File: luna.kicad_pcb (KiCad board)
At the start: 2 copper layers, 85 x 83.8 mm, 31 parts, among them J1 Conn_01x06_Male, J2 Conn_02x12_Top_Bottom, J3 Conn_01x02_Male, J4 Conn_01x02_Male, J5 Screw_Terminal_01x06, Q1 2N7002, Q2 2N7002, Q3 2N7002, Q4 DMN3404L, Q5 DMN3404L, Q6 DMN3404L, U1 LD1117S33TR_SOT223, U2 ESP32-WROOM-32

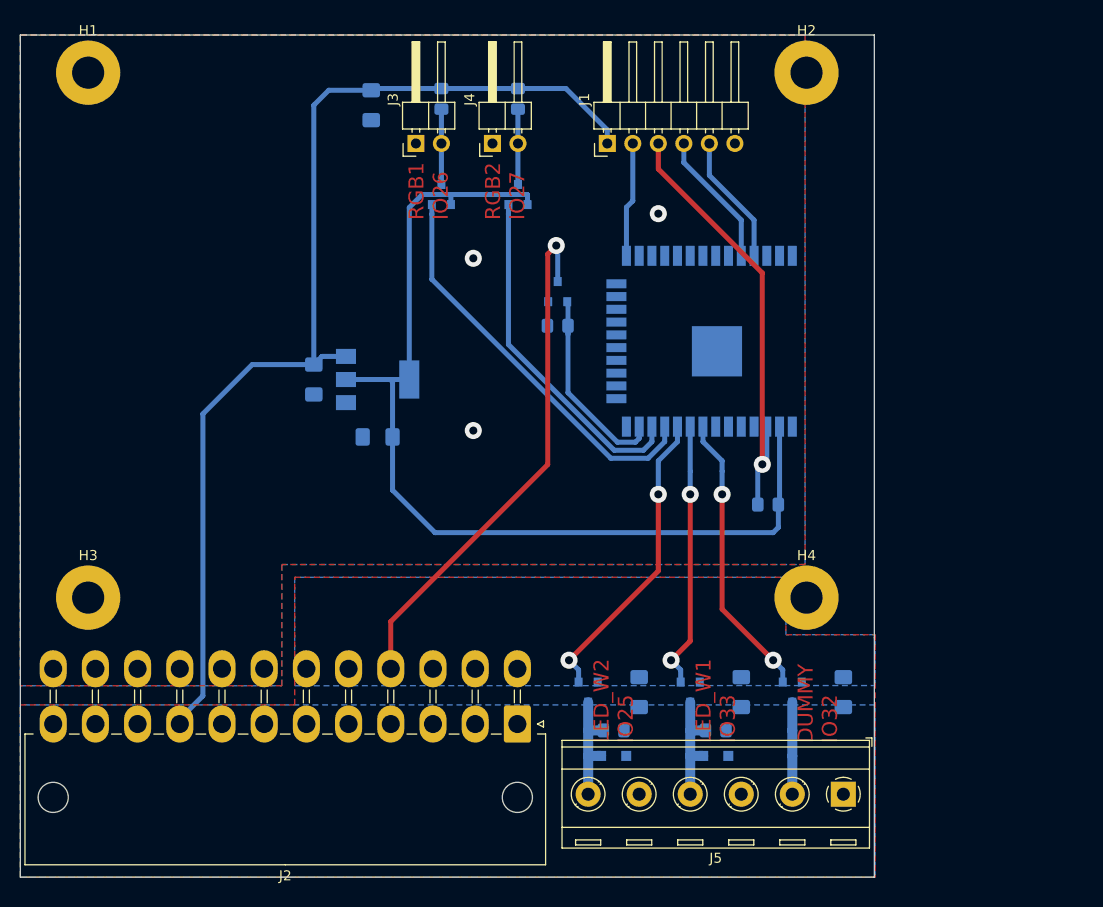
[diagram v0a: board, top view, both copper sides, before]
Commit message: Design in progress.
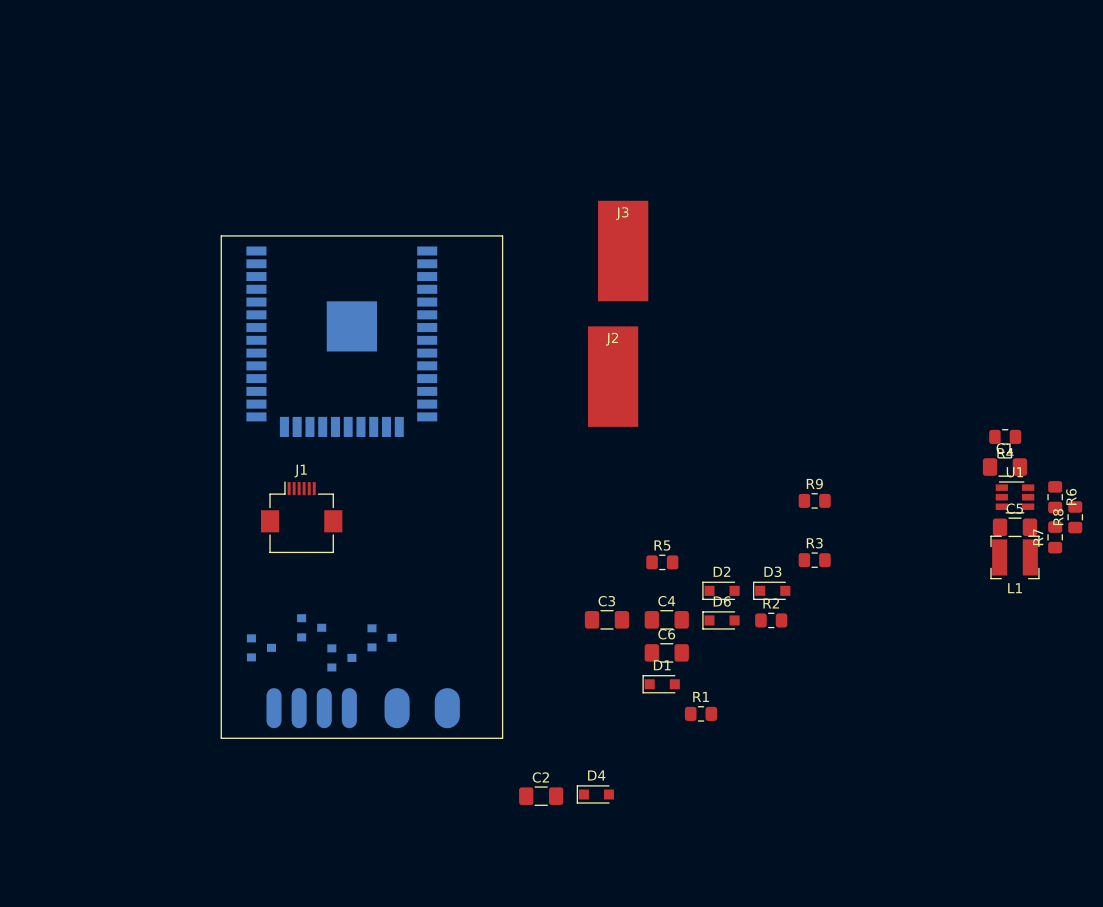
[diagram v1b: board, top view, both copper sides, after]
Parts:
- removed H1, H2, H3, H4: MountingHole_Pad, MountingHole:MountingHole_3.2mm_M3_Pad
- removed J4: Conn_01x02_Male, Connector_PinHeader_2.54mm:PinHeader_1x02_P2.54mm_Horizontal
- removed J5: Screw_Terminal_01x06, TerminalBlock_RND:TerminalBlock_RND_205-00291_1x06_P5.08mm_Horizontal
- removed Q5, Q6: DMN3404L, Package_TO_SOT_SMD:SOT-23
- added D3: D_Schottky, Diode_SMD:D_SOD-323_HandSoldering, F.Cu at (74.9, 55.3)
- added D4: D_Schottky, Diode_SMD:D_SOD-323_HandSoldering, F.Cu at (57.3, 75.6)
- added D5: LED_AGRB, custom:LED_STRIP_RGB, B.Cu at (29.0, 67.0)
- added D6: D_Schottky, Diode_SMD:D_SOD-323_HandSoldering, F.Cu at (69.8, 58.3)
- added D7: LED, custom:LED_STRIP, B.Cu at (40.0, 67.0)
- added L1: 6u5, Inductor_SMD:L_Bourns-SRN4018, F.Cu at (99.0, 52.0)
- added R7: 33k, Resistor_SMD:R_0805_2012Metric_Pad1.15x1.40mm_HandSolder, F.Cu at (103.0, 50.0)
- added R8: 10k, Resistor_SMD:R_0805_2012Metric_Pad1.15x1.40mm_HandSolder, F.Cu at (105.0, 48.0)
- added R9: 10k, Resistor_SMD:R_0805_2012Metric_Pad1.15x1.40mm_HandSolder, F.Cu at (79.1, 46.4)
- C1: value 10u -> 22u; moved to F.Cu
- C2, C3, C4, C6, D1, D2, R2, R5: moved to F.Cu
- C5: value 10u -> 1u; moved to F.Cu
- J1: value Conn_01x06_Male -> Conn_01x06_MountingPin; footprint Connector_PinHeader_2.54mm:PinHeader_1x06_P2.54mm_Horizontal -> Connector_FFC-FPC:Hirose_FH12-6S-0.5SH_1x06-1MP_P0.50mm_Horizontal
- J2: value Conn_02x12_Top_Bottom -> Conn_01x01; footprint Connector_Molex:Molex_Mini-Fit_Jr_5569-24A2_2x12_P4.20mm_Horizontal -> Connector_Wire:SolderWirePad_1x01_SMD_5x10mm
- J3: value Conn_01x02_Male -> Conn_01x01; footprint Connector_PinHeader_2.54mm:PinHeader_1x02_P2.54mm_Horizontal -> Connector_Wire:SolderWirePad_1x01_SMD_5x10mm
- Q1, Q2, Q3: value 2N7002 -> DMN3404L
- R1, R3: value 1k -> 10k; moved to F.Cu
- R4: value 10k -> 100k; moved to F.Cu
- R6: value 10k -> 47k; moved to F.Cu
- U1: value LD1117S33TR_SOT223 -> AP65111AWU; footprint Package_TO_SOT_SMD:SOT-223-3_TabPin2 -> Package_TO_SOT_SMD:TSOT-23-6; moved to F.Cu
- moved C1 72.6 mm to (98.0, 43.0), turned to 0 degrees
- moved R1 66.4 mm to (67.8, 67.6), turned to 0 degrees
- moved U1 64.5 mm to (99.0, 46.0)
- moved R3 54.6 mm to (79.1, 52.3), turned to 0 degrees
- moved R6 49.7 mm to (103.0, 46.0), turned to 270 degrees
- moved Q3 49.3 mm to (32.0, 62.0), turned to 0 degrees
- moved J1 47.3 mm to (28.0, 47.0), turned to 0 degrees
- moved C2 47.2 mm to (51.8, 75.8), turned to 0 degrees
- moved Q2 46.1 mm to (24.0, 61.0), turned to 0 degrees
- moved Q1 45.0 mm to (29.0, 59.0), turned to 0 degrees
- moved Q4 41.2 mm to (36.0, 60.0), turned to 0 degrees
- moved U2 36.6 mm to (32.0, 29.8), turned to 180 degrees
- moved R2 36.2 mm to (74.7, 58.3), turned to 0 degrees
- moved J2 35.9 mm to (59.0, 34.0), turned to 0 degrees
- moved C5 31.8 mm to (99.0, 49.0), turned to 0 degrees
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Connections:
- net DUMMY_LOAD renamed LED_W
- net Net-(J4-Pad2) renamed LED_B_OUT
- C1 pad 1: +5V -> +12V
- C2 pad 1: GND -> +12V
- C2 pad 2: +5V -> GND
- C3 pad 1: VDD -> +12V
- C4 pad 2: GNDPWR -> GND
- C5 pad 1: +12V -> Net-(C5-Pad1)
- C5 pad 2: GNDPWR -> Net-(C5-Pad2)
- C6 pad 2: GNDPWR -> GND
- D1 pad 2: LED_W1_OUT -> LED_R_OUT
- D2 pad 2: LED_W2_OUT -> LED_G_OUT
- J2 pad 1: Net-(J2-Pad1) -> +12V
- Q1 pad 1: VDD -> LED_R
- Q1 pad 2: RGB1 -> GND
- Q1 pad 3: Net-(J3-Pad2) -> LED_R_OUT
- Q2 pad 1: ~ON~ -> LED_G
- Q2 pad 3: Net-(J2-Pad16) -> LED_G_OUT
- Q3 pad 1: VDD -> LED_B
- Q3 pad 2: RGB2 -> GND
- Q4 pad 2: GNDPWR -> GND
- Q4 pad 3: DUMMY_LOAD_OUT -> Net-(D6-Pad2)
- R1 pad 1: +5V -> +12V
- R1 pad 2: Net-(J3-Pad2) -> LED_R_OUT
- R2 pad 1: ~ON~ -> +12V
- R2 pad 2: GND -> LED_G_OUT
- R3 pad 1: +5V -> +12V
- R4 pad 1: VDD -> Net-(R4-Pad1)
- R4 pad 2: EN -> +12V
- R5 pad 2: LED_W1_OUT -> Net-(D6-Pad2)
- R6 pad 1: +12V -> Net-(R6-Pad1)
- R6 pad 2: LED_W2_OUT -> Net-(R6-Pad2)
- U1 pad 1: GND -> +12V
- U1 pad 2: VDD -> GND
- U1 pad 3: +5V -> Net-(C5-Pad1)
- U2 pad 10: LED_W2 -> LED_G
- U2 pad 11: RGB1 -> LED_B
- U2 pad 12: RGB2 -> Net-(U2-Pad12)
- U2 pad 13: ~ON~ -> Net-(U2-Pad13)
- U2 pad 9: LED_W1 -> LED_R
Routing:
- net +5V: track 107.2 -> 0.00 mm
- net VDD: track 99.5 -> 0.00 mm
- net Net-(J2-Pad16): track 51.1 -> 0.00 mm, vias 1 -> 0
- net EN: track 44.4 -> 0.00 mm, vias 1 -> 0
- net RGB1: track 40.2 -> 0.00 mm
- net RGB2: track 34.4 -> 0.00 mm
- net LED_W2: track 30.3 -> 0.00 mm, vias 2 -> 0
- net LED_W: track 28.7 -> 0.00 mm, vias 2 -> 0
- net LED_W1: track 26.6 -> 0.00 mm, vias 2 -> 0
- net ~ON~: track 19.5 -> 0.00 mm
- net RX: track 13.6 -> 0.00 mm
- net TX: track 13.0 -> 0.00 mm
- net LED_W1_OUT: track 12.0 -> 0.00 mm
- net LED_W2_OUT: track 12.0 -> 0.00 mm
- net BOOT: track 11.4 -> 0.00 mm
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- removed copper zone on B.Cu, net +12V
- removed copper zone on B.Cu, net GND
- removed copper zone on F.Cu, net GND
- removed copper zone on B.Cu, net GNDPWR
- removed copper zone on F.Cu, net GNDPWR
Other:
- board outline removed
- board text removed: "DUMMY IO32"
- board text removed: "LED_W1 IO33"
- board text removed: "LED_W2 IO25"
- board text removed: "RGB1 IO26"
- board text removed: "RGB2 IO27"
